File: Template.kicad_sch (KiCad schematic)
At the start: 22 parts, among them J1 OLED, SW1 SW_Push, U1 ProMicro

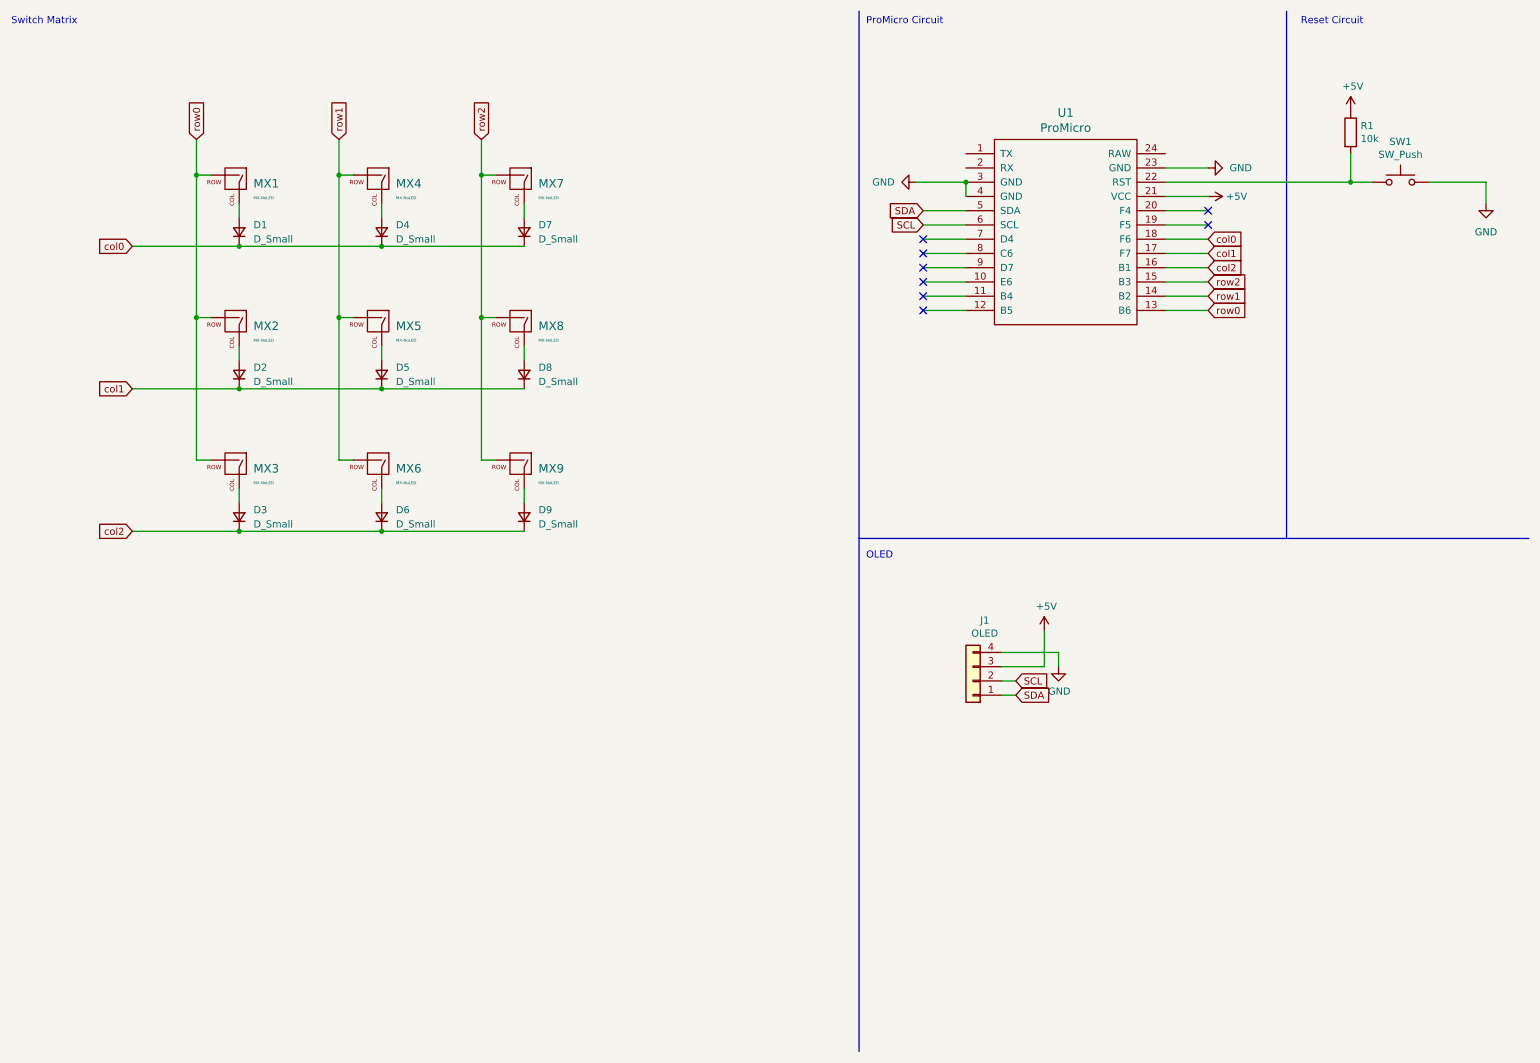
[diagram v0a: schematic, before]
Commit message: Reset to blank
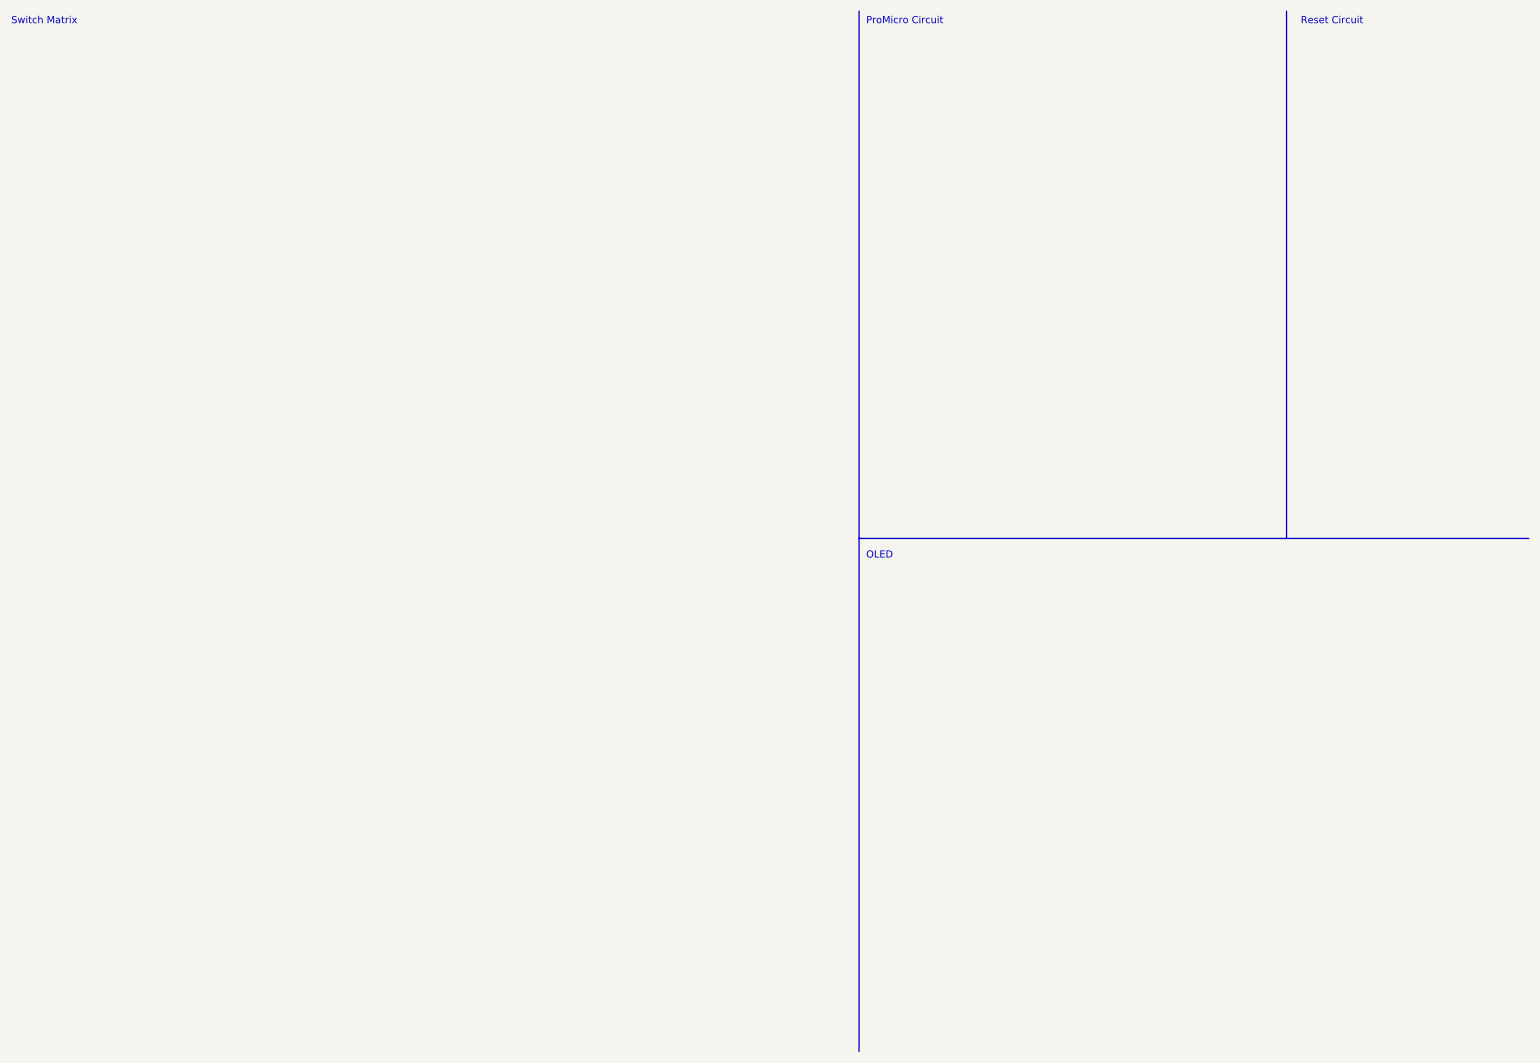
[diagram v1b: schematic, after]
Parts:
- removed D1, D2, D3, D4, D5, D6, D7, D8, D9: D_Small, bevin:D3_TH_nonHybrid, symbol Device:D_Small
- removed J1: OLED, bevin:OLED_v2, symbol Connector_Generic:Conn_01x04
- removed MX1, MX2, MX3, MX4, MX5, MX6, MX7, MX8, MX9: MX-NoLED, bevin:MXOnly-1U-NoLED, symbol mx:MX-NoLED
- removed R1: 10k, bevin:R3_TH_nonHybrid, symbol Device:R
- removed SW1: SW_Push, Button_Switch_SMD:SW_SPST_TL3342, symbol Switch:SW_Push
- removed U1: ProMicro, bevin:ProMicro_v3, symbol promicro:ProMicro
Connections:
- no-connect marks 8 -> 0
